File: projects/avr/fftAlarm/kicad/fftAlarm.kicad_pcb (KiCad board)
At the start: 2 copper layers, 76.2 x 35.6 mm, 29 parts, among them P1 CONN_1, P2 CONN_1, P3 CONN_1, P5 CONN_6, Q1 NPN, Q2 NPN, U1 ATTINY85-20PU, U2 7805

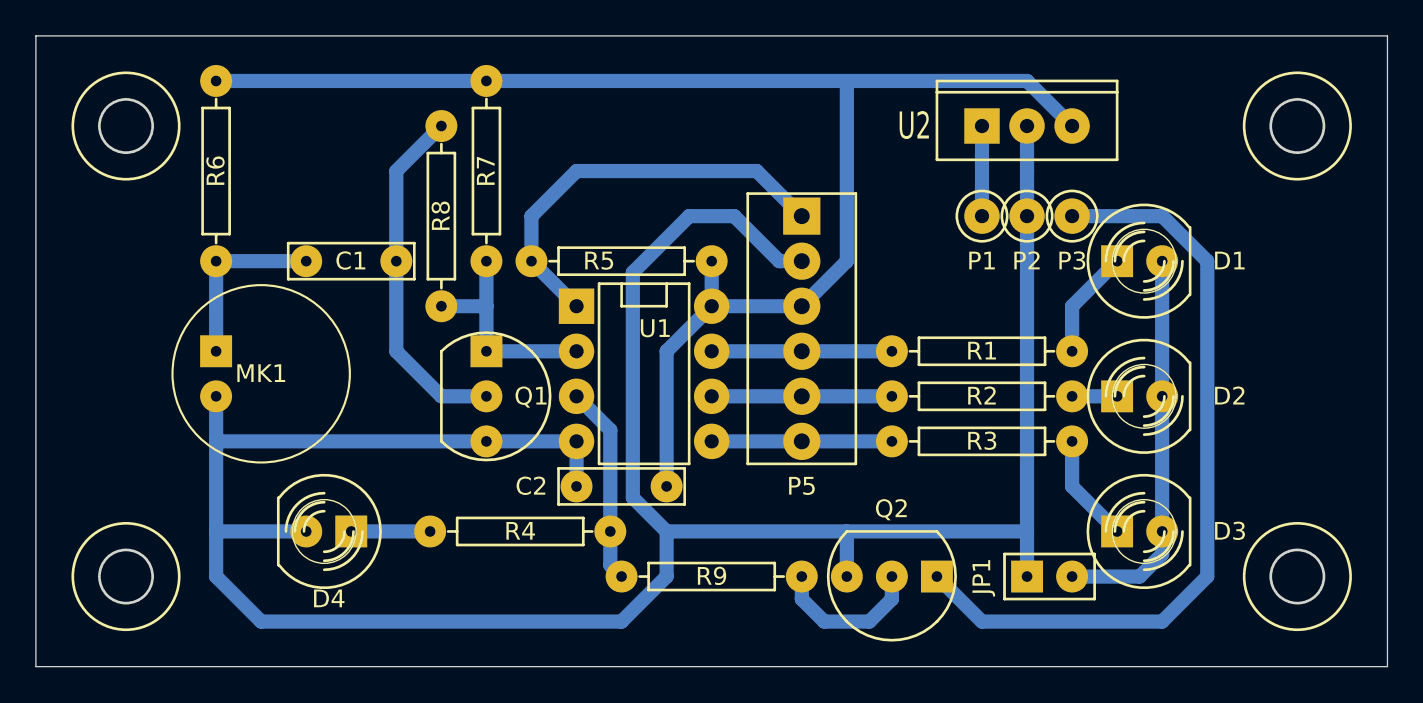
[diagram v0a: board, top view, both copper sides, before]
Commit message: update kicad files
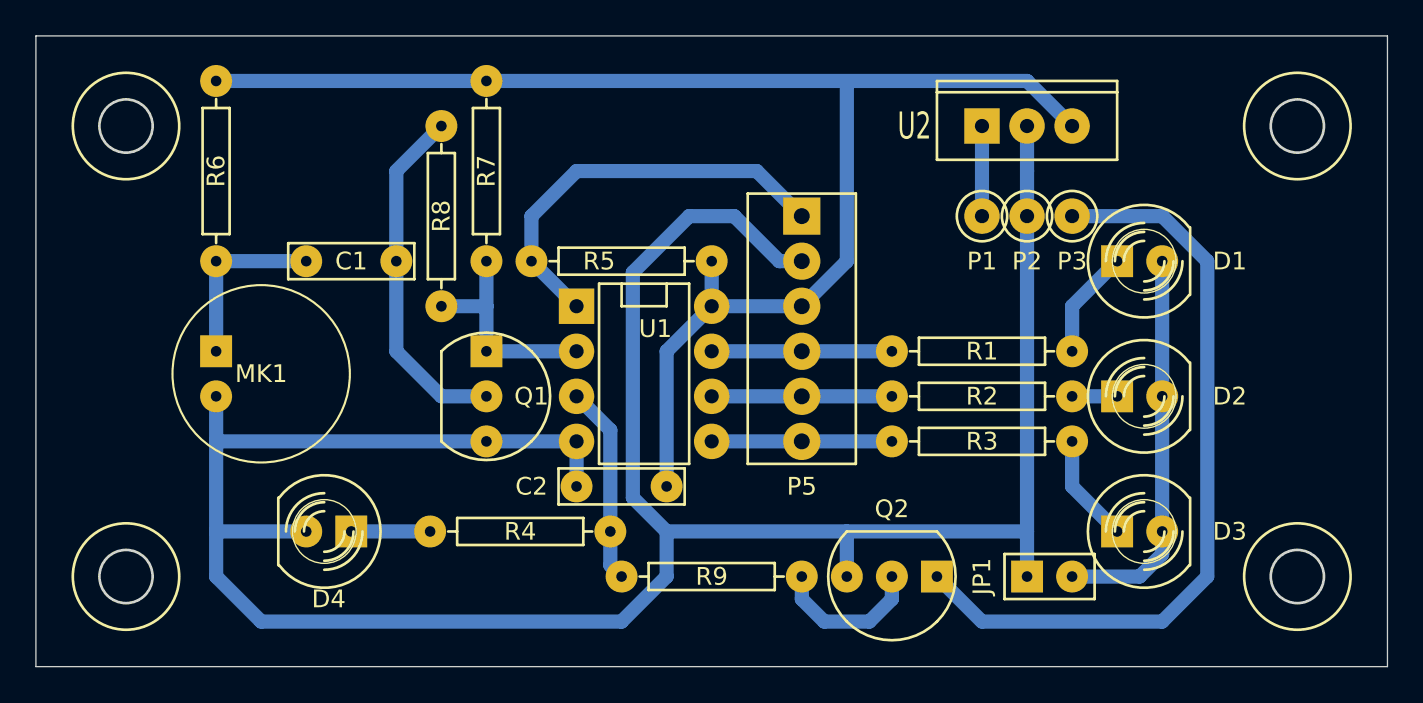
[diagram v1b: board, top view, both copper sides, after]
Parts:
- C1, C2: footprint kicad:C2 -> common:C2
- D1, D2, D3, D4: footprint kicad:LED-5MM -> common:LED-5MM
- JP1: footprint kicad:PIN_ARRAY_2X1 -> common:PIN_ARRAY_2X1
- MK1: footprint kicad:ELECTRET -> common:ELECTRET
- P1, P2, P3: footprint kicad:PIN_ARRAY_1X1 -> common:PIN_ARRAY_1X1
- P5: footprint kicad:PIN_ARRAY_6X1 -> common:PIN_ARRAY_6X1
- Q1, Q2: footprint kicad:NPN -> common:NPN
- R1, R2, R3, R4, R5, R6, R7, R8, R9: footprint kicad:R4 -> common:R4
- REF** (x4): footprint kicad:ENTRETOISE -> common:ENTRETOISE
- U1: footprint kicad:DIP-8__300 -> common:DIP-8__300
- U2: footprint kicad:TO220_VERT -> common:TO220_VERT
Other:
- net class Default removed
